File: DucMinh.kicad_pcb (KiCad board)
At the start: 2 copper layers, 90 x 80 mm, 62 parts, among them J1 Power, J10 HC05, J11 PWR_Selection, J12 BOOT0, J2 M1, J3 USB_B_Micro, J4 M2, J5 M3, J6 AS5600, J7 STLink, J8 Stepper_Motor, SW1 SW_Push, U10 BTS7960B, U2 AMS1117-3.3, U3 LM2596SX-5.0/NOPB, U4 TMC2209_SILENTSTEPSTICK, U5 BTS7960B, U6 STM32F103RCT6, U8 BTS7960B, Y1 8 MHz

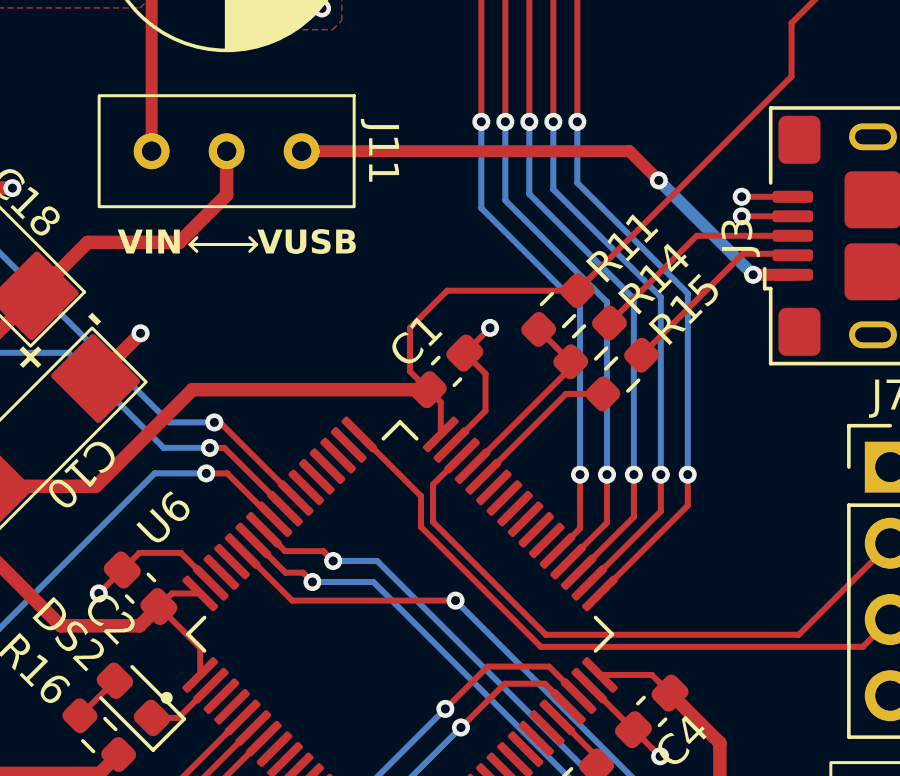
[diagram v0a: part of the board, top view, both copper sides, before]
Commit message: final2
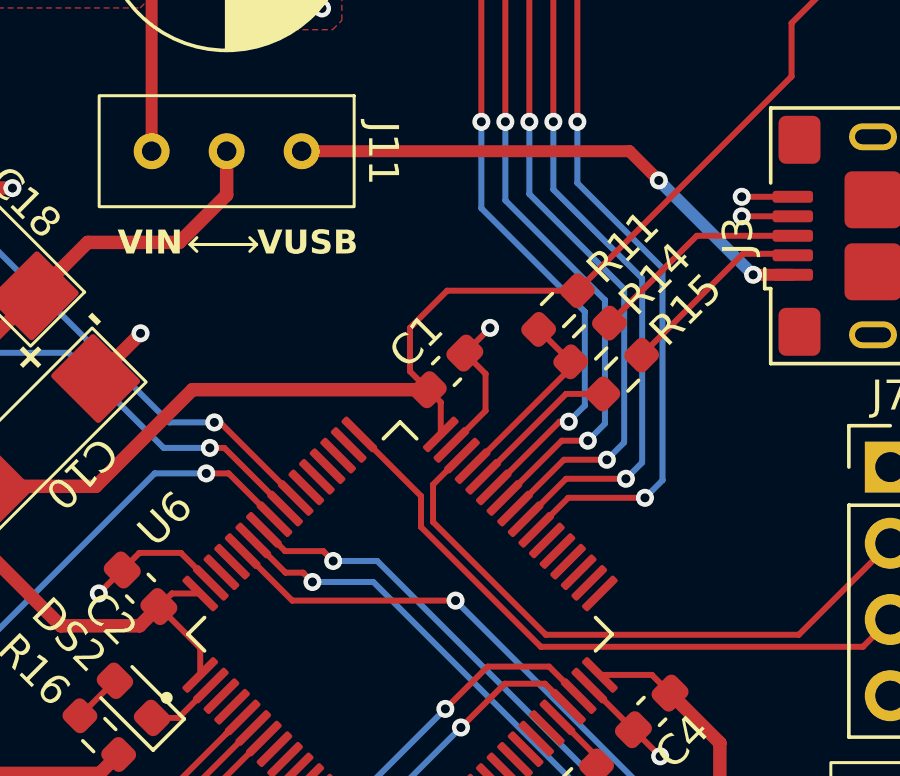
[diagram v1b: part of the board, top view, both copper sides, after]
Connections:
- U6 pad 33: DIR_PIN -> unconnected-(U6-PB12-Pad33)
- U6 pad 34: STEP_PIN -> unconnected-(U6-PB13-Pad34)
- U6 pad 35: MS2_PIN -> unconnected-(U6-PB14-Pad35)
- U6 pad 36: MS1_PIN -> unconnected-(U6-PB15-Pad36)
- U6 pad 37: ENABLE_PIN -> unconnected-(U6-PC6-Pad37)
- U6 pad 39: unconnected-(U6-PC8-Pad39) -> DIR_PIN
- U6 pad 40: unconnected-(U6-PC9-Pad40) -> STEP_PIN
- U6 pad 41: unconnected-(U6-PA8-Pad41) -> MS2_PIN
- U6 pad 42: unconnected-(U6-PA9-Pad42) -> MS1_PIN
- U6 pad 43: unconnected-(U6-PA10-Pad43) -> ENABLE_PIN
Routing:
- net ENABLE_PIN: track 32.6 -> 31.6 mm
- net MS1_PIN: track 32.6 -> 31.7 mm
- net MS2_PIN: track 32.4 -> 31.7 mm
- net STEP_PIN: track 35.8 -> 35.1 mm
